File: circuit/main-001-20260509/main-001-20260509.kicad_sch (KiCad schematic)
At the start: 20 parts, among them J1 Conn_Relay, J2 Conn_Sub, Q1 BSS138, Q2 BSS138, SW1 RESET, U1 DEV-16771, U2 BNO055

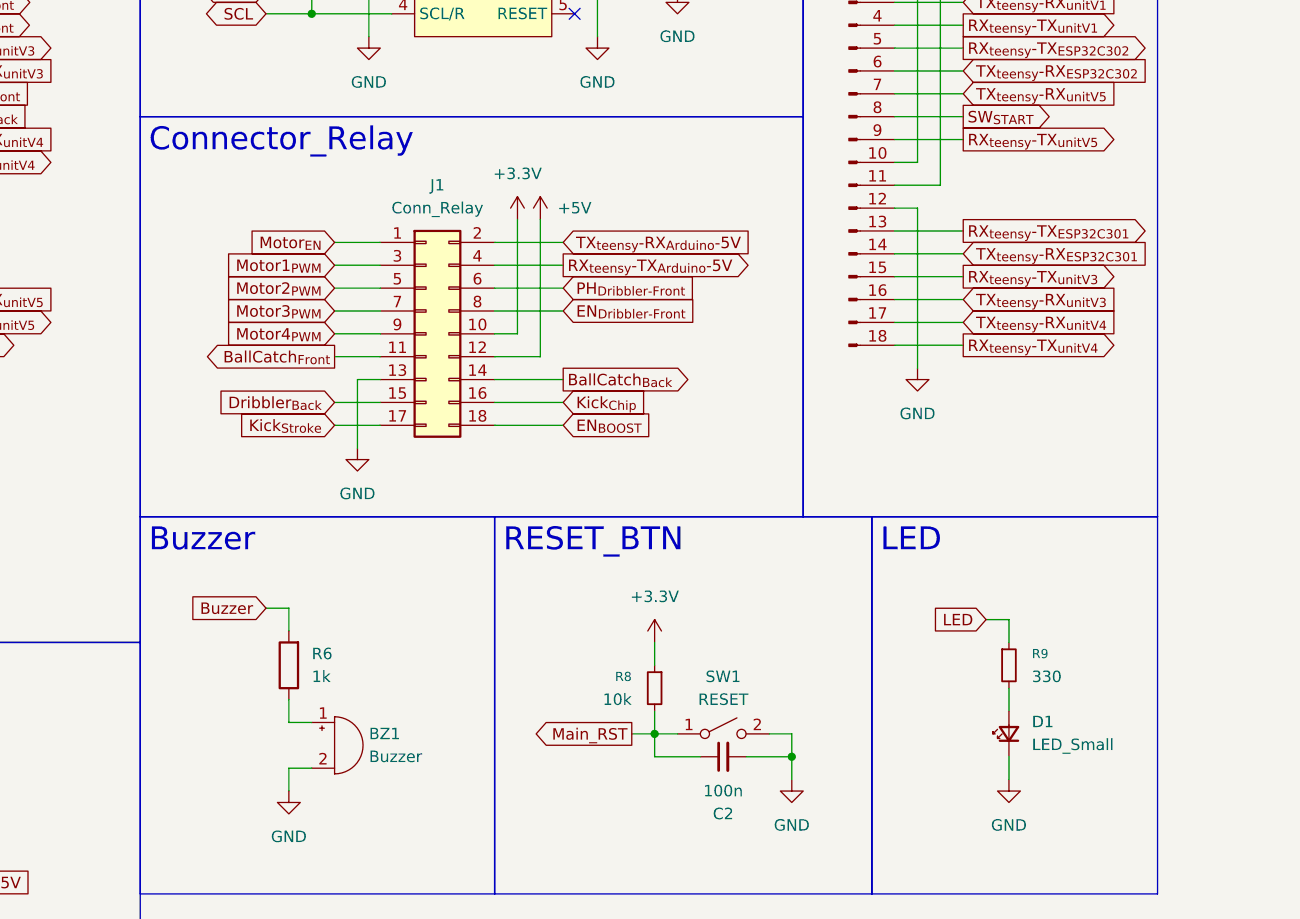
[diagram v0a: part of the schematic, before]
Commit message: Update メイン基板の修正を完了させた
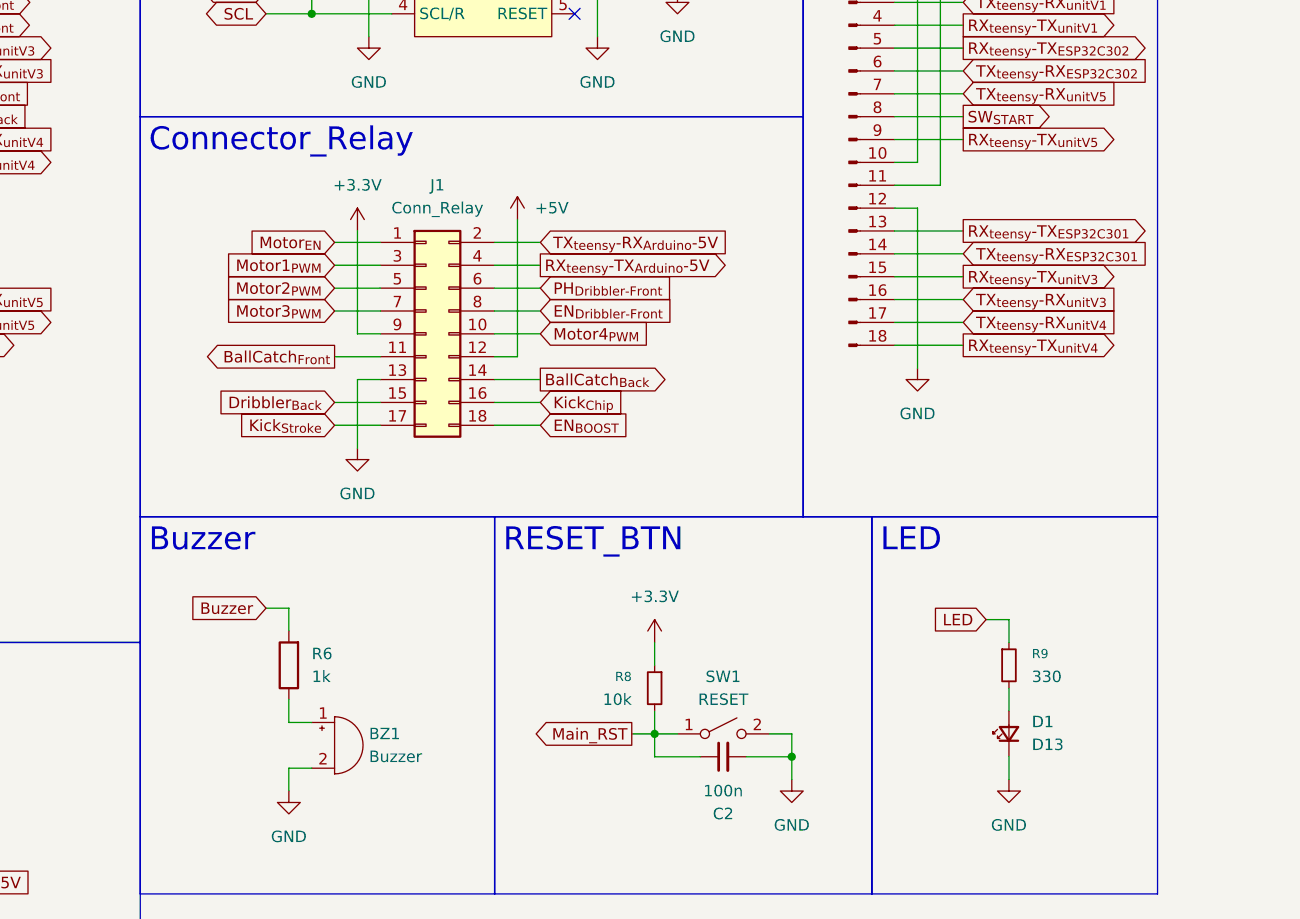
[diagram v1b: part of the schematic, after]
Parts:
- D1: value LED_Small -> D13
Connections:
- net +3.3V: now also J1.9 (Pin_9); no longer J1.10 (Pin_10)
- net Motor4_{PWM}: now also J1.10 (Pin_10); no longer J1.9 (Pin_9)
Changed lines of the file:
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@@
 	(wire
 		(pts
-			(xy 144.78 71.12) (xy 137.16 71.12)
-		)
-		(stroke
-			(width 0)
-			(type default)
-		)
-	)
-	(wire
-		(pts
 			(xy 46.99 165.1) (xy 46.99 167.64)
 		)
@@
 	(wire
 		(pts
-			(xy 142.24 63.5) (xy 142.24 78.74)
+			(xy 139.7 63.5) (xy 139.7 78.74)
 		)
 		(stroke
@@
 	(wire
 		(pts
+			(xy 121.92 76.2) (xy 124.46 76.2)
+		)
+		(stroke
+			(width 0)
+			(type default)
+		)
+	)
+	(wire
+		(pts
 			(xy 68.58 39.37) (xy 71.12 39.37)
 		)
@@
 	(wire
 		(pts
-			(xy 144.78 86.36) (xy 137.16 86.36)
+			(xy 142.24 86.36) (xy 137.16 86.36)
 		)
 		(stroke
@@
 	(wire
 		(pts
-			(xy 137.16 81.28) (xy 144.78 81.28)
+			(xy 137.16 81.28) (xy 142.24 81.28)
 		)
 		(stroke
@@
 	(wire
 		(pts
+			(xy 137.16 73.66) (xy 142.24 73.66)
+		)
+		(stroke
+			(width 0)
+			(type default)
+		)
+	)
+	(wire
+		(pts
 			(xy 38.1 74.93) (xy 40.64 74.93)
 		)
@@
 	(wire
 		(pts
-			(xy 144.78 83.82) (xy 137.16 83.82)
+			(xy 142.24 83.82) (xy 137.16 83.82)
 		)
 		(stroke
@@
 	(wire
 		(pts
-			(xy 144.78 66.04) (xy 137.16 66.04)
-		)
-		(stroke
-			(width 0)
-			(type default)
-		)
-	)
-	(wire
-		(pts
-			(xy 144.78 73.66) (xy 137.16 73.66)
-		)
-		(stroke
-			(width 0)
-			(type default)
-		)
-	)
-	(wire
-		(pts
 			(xy 194.31 107.95) (xy 194.31 110.49)
 		)
@@
 	(wire
 		(pts
-			(xy 142.24 78.74) (xy 137.16 78.74)
+			(xy 139.7 78.74) (xy 137.16 78.74)
 		)
 		(stroke
@@
 	(wire
 		(pts
-			(xy 144.78 68.58) (xy 137.16 68.58)
-		)
-		(stroke
-			(width 0)
-			(type default)
-		)
-	)
-	(wire
-		(pts
 			(xy 68.58 46.99) (xy 71.12 46.99)
 		)
@@
 	(wire
 		(pts
-			(xy 38.1 64.77) (xy 40.64 64.77)
+			(xy 121.92 64.77) (xy 121.92 76.2)
 		)
 		(stroke
@@
 	(wire
 		(pts
-			(xy 139.7 63.5) (xy 139.7 76.2)
+			(xy 38.1 64.77) (xy 40.64 64.77)
 		)
 		(stroke
@@
 	(wire
 		(pts
+			(xy 137.16 71.12) (xy 142.24 71.12)
+		)
+		(stroke
+			(width 0)
+			(type default)
+		)
+	)
+	(wire
+		(pts
 			(xy 111.76 38.1) (xy 114.3 38.1)
 		)
@@
 	(wire
 		(pts
+			(xy 137.16 66.04) (xy 142.24 66.04)
+		)
+		(stroke
+			(width 0)
+			(type default)
+		)
+	)
+	(wire
+		(pts
 			(xy 68.58 41.91) (xy 71.12 41.91)
 		)
@@
 	(wire
 		(pts
-			(xy 119.38 76.2) (xy 124.46 76.2)
-		)
-		(stroke
-			(width 0)
-			(type default)
-		)
-	)
-	(wire
-		(pts
 			(xy 189.23 72.39) (xy 181.61 72.39)
 		)
@@
 	(wire
 		(pts
-			(xy 139.7 76.2) (xy 137.16 76.2)
+			(xy 137.16 76.2) (xy 142.24 76.2)
 		)
 		(stroke
@@
 	(wire
 		(pts
+			(xy 137.16 68.58) (xy 142.24 68.58)
+		)
+		(stroke
+			(width 0)
+			(type default)
+		)
+	)
+	(wire
+		(pts
 			(xy 68.58 64.77) (xy 71.12 64.77)
 		)
@@
 	(global_label "Motor4_{PWM}"
 		(shape input)
-		(at 119.38 76.2 180)
+		(at 142.24 76.2 0)
 		(fields_autoplaced yes)
 		(effects
@@
 				(size 1.27 1.27)
 			)
-			(justify right)
+			(justify left)
 		)
 		(property "Intersheetrefs" "${INTERSHEET_REFS}"
-			(at 106.535 76.2 0)
+			(at 155.085 76.2 0)
 			(hide yes)
 			(show_name no)
@@
 					(size 1.27 1.27)
 				)
-				(justify right)
+				(justify left)
 			)
 		)
@@
 	(global_label "EN_{BOOST}"
 		(shape input)
-		(at 144.78 86.36 0)
+		(at 142.24 86.36 0)
 		(fields_autoplaced yes)
 		(effects
@@
 		)
 		(property "Intersheetrefs" "${INTERSHEET_REFS}"
-			(at 155.182 86.36 0)
+			(at 152.642 86.36 0)
 			(hide yes)
 			(show_name no)
@@
 	(global_label "BallCatch_{Back}"
 		(shape output)
-		(at 144.78 81.28 0)
+		(at 142.24 81.28 0)
 		(fields_autoplaced yes)
 		(effects
@@
 		)
 		(property "Intersheetrefs" "${INTERSHEET_REFS}"
-			(at 157.6722 81.28 0)
+			(at 155.1322 81.28 0)
 			(hide yes)
 			(show_name no)
@@
 	(global_label "RX_{teensy}-TX_{Arduino}-5V"
 		(shape output)
-		(at 144.78 68.58 0)
+		(at 142.24 68.58 0)
 		(fields_autoplaced yes)
 		(effects
@@
 		)
 		(property "Intersheetrefs" "${INTERSHEET_REFS}"
-			(at 168.3634 68.58 0)
+			(at 165.8234 68.58 0)
 			(hide yes)
 			(show_name no)
@@
 	(global_label "PH_{Dribbler-Front}"
 		(shape input)
-		(at 144.78 71.12 0)
+		(at 142.24 71.12 0)
 		(fields_autoplaced yes)
 		(effects
@@
 		)
 		(property "Intersheetrefs" "${INTERSHEET_REFS}"
-			(at 157.0233 71.12 0)
+			(at 154.4833 71.12 0)
 			(hide yes)
 			(show_name no)
@@
 	(global_label "TX_{teensy}-RX_{Arduino}-5V"
 		(shape input)
-		(at 144.78 66.04 0)
+		(at 142.24 66.04 0)
 		(fields_autoplaced yes)
 		(effects
@@
 		)
 		(property "Intersheetrefs" "${INTERSHEET_REFS}"
-			(at 168.3634 66.04 0)
+			(at 165.8234 66.04 0)
 			(hide yes)
 			(show_name no)
@@
 	(global_label "EN_{Dribbler-Front}"
 		(shape input)
-		(at 144.78 73.66 0)
+		(at 142.24 73.66 0)
 		(fields_autoplaced yes)
 		(effects
@@
 		)
 		(property "Intersheetrefs" "${INTERSHEET_REFS}"
-			(at 157.0233 73.66 0)
+			(at 154.4833 73.66 0)
 			(hide yes)
 			(show_name no)
@@
 	(global_label "Kick_{Chip}"
 		(shape input)
-		(at 144.78 83.82 0)
+		(at 142.24 83.82 0)
 		(fields_autoplaced yes)
 		(effects
@@
 		)
 		(property "Intersheetrefs" "${INTERSHEET_REFS}"
-			(at 153.2378 83.82 0)
+			(at 150.6978 83.82 0)
 			(hide yes)
 			(show_name no)
@@
 	(symbol
 		(lib_id "power:+5V")
-		(at 142.24 63.5 0)
+		(at 139.7 63.5 0)
 		(unit 1)
 		(body_style 1)
@@
 		(dnp no)
 		(property "Reference" "#PWR020"
-			(at 142.24 67.31 0)
+			(at 139.7 67.31 0)
 			(hide yes)
 			(show_name no)
@@
 		)
 		(property "Value" "+5V"
-			(at 146.05 62.23 0)
+			(at 143.51 62.23 0)
 			(show_name no)
 			(do_not_autoplace no)
@@
 		)
 		(property "Footprint" ""
-			(at 142.24 63.5 0)
+			(at 139.7 63.5 0)
 			(hide yes)
 			(show_name no)
@@
 		)
 		(property "Datasheet" ""
-			(at 142.24 63.5 0)
+			(at 139.7 63.5 0)
 			(hide yes)
 			(show_name no)
@@
 		)
 		(property "Description" "Power symbol creates a global label with name \"+5V\""
-			(at 142.24 63.5 0)
+			(at 139.7 63.5 0)
 			(hide yes)
 			(show_name no)
@@
 	(symbol
 		(lib_id "power:+3.3V")
-		(at 139.7 63.5 0)
+		(at 121.92 64.77 0)
 		(unit 1)
 		(body_style 1)
@@
 		(fields_autoplaced yes)
 		(property "Reference" "#PWR010"
-			(at 139.7 67.31 0)
+			(at 121.92 68.58 0)
 			(hide yes)
 			(show_name no)
@@
 		)
 		(property "Value" "+3.3V"
-			(at 139.7 58.42 0)
+			(at 121.92 59.69 0)
 			(show_name no)
 			(do_not_autoplace no)
@@
 		)
 		(property "Footprint" ""
-			(at 139.7 63.5 0)
+			(at 121.92 64.77 0)
 			(hide yes)
 			(show_name no)
@@
 		)
 		(property "Datasheet" ""
-			(at 139.7 63.5 0)
+			(at 121.92 64.77 0)
 			(hide yes)
 			(show_name no)
@@
 		)
 		(property "Description" "Power symbol creates a global label with name \"+3.3V\""
-			(at 139.7 63.5 0)
+			(at 121.92 64.77 0)
 			(hide yes)
 			(show_name no)
@@
 			)
 		)
-		(property "Value" "LED_Small"
+		(property "Value" "D13"
 			(at 196.85 121.8564 90)
 			(show_name no)
